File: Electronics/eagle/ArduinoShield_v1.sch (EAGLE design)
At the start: 41 parts, among them IC1 74AC14N, IC3 ACS770LCB-50B

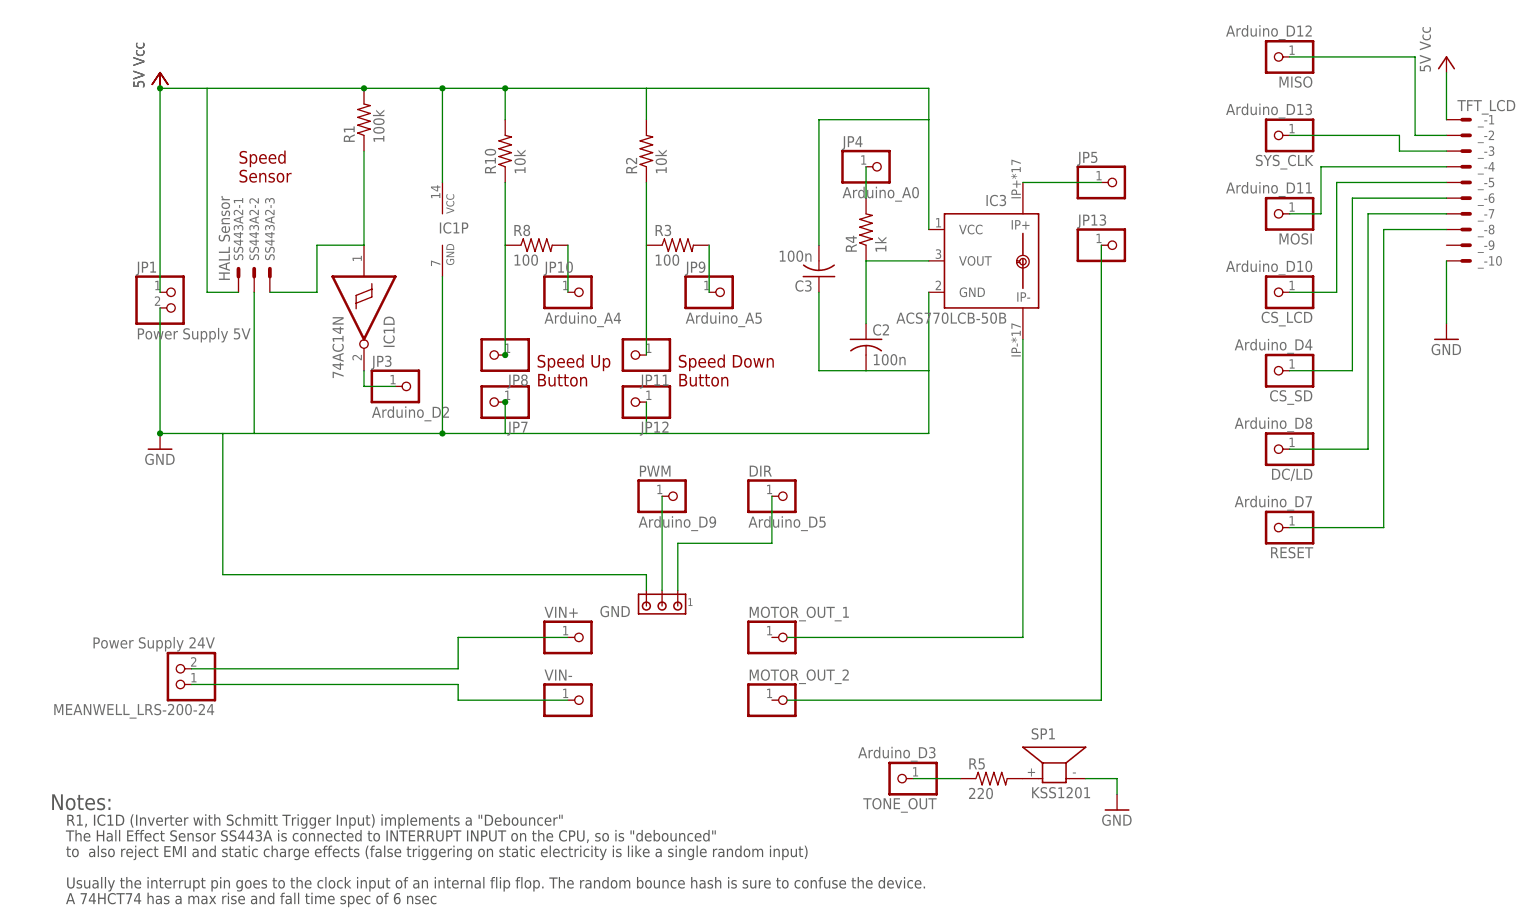
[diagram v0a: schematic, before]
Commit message: Version 0.9
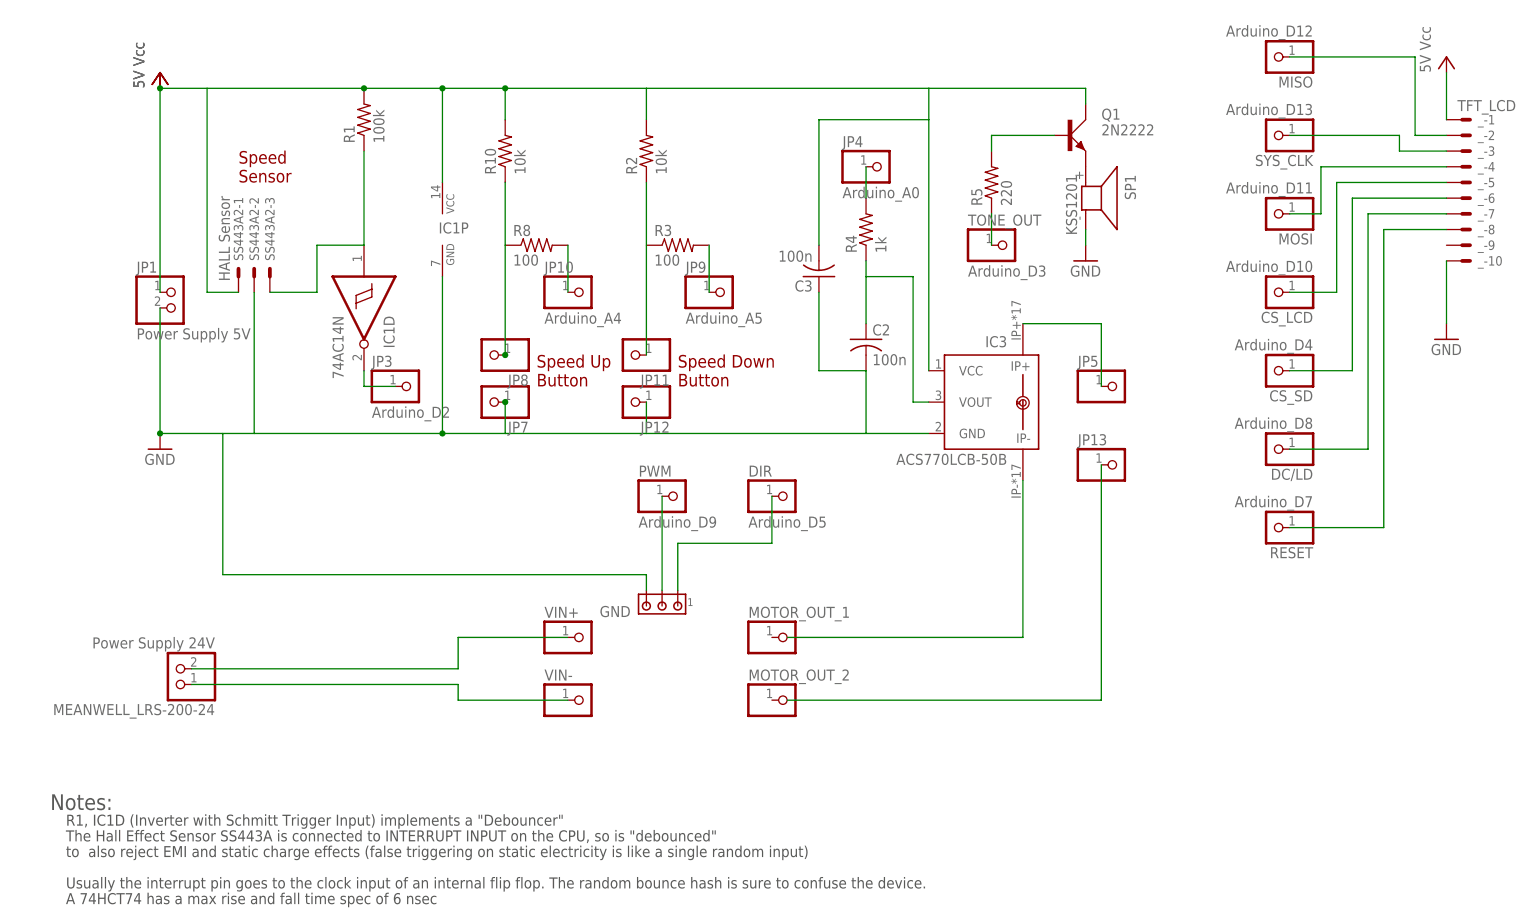
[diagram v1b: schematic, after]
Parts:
- added Q1: 2N2222, transistor-small-signal:2N2222
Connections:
- new net N$23: Q1.B, R5.2
- net N$14: now also Q1.E; no longer R5.2
- net VCC: now also Q1.C
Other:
- moved on the sheet: IC3, JP13, JP5, R5, SP1, TONE_OUT
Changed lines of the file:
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@@
 <part name="RESET" library="pinhead" deviceset="PINHD-1X1" device="" value="Arduino_D7"/>
 <part name="GND3" library="supply1" deviceset="GND" device=""/>
+<part name="Q1" library="transistor-small-signal" deviceset="2N2222" device=""/>
 </parts>
 <sheets>
@@
 <text x="109.22" y="63.5" size="3.81" layer="90">  Motor
 Controller</text>
-<text x="190.5" y="139.7" size="3.81" layer="90" align="center">  Motor
+<text x="190.5" y="106.68" size="3.81" layer="90" align="center">  Motor
 </text>
 </plain>
@@
 <instance part="JP12" gate="G$1" x="114.3" y="111.76" rot="R180"/>
 <instance part="R3" gate="G$1" x="121.92" y="137.16"/>
-<instance part="IC3" gate="G$1" x="172.72" y="134.62" rot="MR0"/>
+<instance part="IC3" gate="G$1" x="172.72" y="111.76" rot="MR0"/>
 <instance part="R4" gate="G$1" x="152.4" y="139.7" rot="R90"/>
 <instance part="JP4" gate="G$1" x="154.94" y="149.86"/>
-<instance part="JP5" gate="G$1" x="193.04" y="147.32"/>
-<instance part="JP13" gate="G$1" x="193.04" y="137.16"/>
+<instance part="JP5" gate="G$1" x="193.04" y="114.3"/>
+<instance part="JP13" gate="G$1" x="193.04" y="101.6"/>
 <instance part="MOTOR_OUT_1" gate="G$1" x="139.7" y="73.66"/>
 <instance part="MOTOR_OUT_2" gate="G$1" x="139.7" y="63.5"/>
@@
 <instance part="PWM" gate="G$1" x="121.92" y="96.52"/>
 <instance part="MEANWELL_LRS-200-24" gate="G$1" x="40.64" y="68.58" rot="R180"/>
-<instance part="SP1" gate="1" x="182.88" y="50.8"/>
+<instance part="SP1" gate="1" x="187.96" y="144.78" rot="R270"/>
 <instance part="P+2" gate="VCC" x="38.1" y="165.1"/>
-<instance part="GND2" gate="1" x="193.04" y="45.72"/>
-<instance part="R5" gate="G$1" x="172.72" y="50.8"/>
-<instance part="TONE_OUT" gate="G$1" x="157.48" y="50.8" rot="R180"/>
+<instance part="GND2" gate="1" x="187.96" y="134.62"/>
+<instance part="R5" gate="G$1" x="172.72" y="147.32" rot="R90"/>
+<instance part="TONE_OUT" gate="G$1" x="175.26" y="137.16"/>
 <instance part="_" gate="-1" x="248.92" y="157.48"/>
 <instance part="_" gate="-2" x="248.92" y="154.94"/>
@@
 <instance part="RESET" gate="G$1" x="218.44" y="91.44" rot="R180"/>
 <instance part="GND3" gate="1" x="246.38" y="121.92"/>
+<instance part="Q1" gate="1" x="185.42" y="154.94"/>
 </instances>
 <busses>
@@
 <wire x1="116.84" y1="157.48" x2="116.84" y2="162.56" width="0.1524" layer="91"/>
 <pinref part="IC3" gate="G$1" pin="VCC"/>
-<wire x1="162.56" y1="139.7" x2="162.56" y2="157.48" width="0.1524" layer="91"/>
+<wire x1="162.56" y1="116.84" x2="162.56" y2="157.48" width="0.1524" layer="91"/>
 <pinref part="C3" gate="G$1" pin="2"/>
 <wire x1="162.56" y1="157.48" x2="162.56" y2="162.56" width="0.1524" layer="91"/>
@@
 <junction x="71.12" y="162.56"/>
 <pinref part="P+2" gate="VCC" pin="VCC"/>
+<wire x1="162.56" y1="162.56" x2="187.96" y2="162.56" width="0.1524" layer="91"/>
+<pinref part="Q1" gate="1" pin="C"/>
+<wire x1="187.96" y1="162.56" x2="187.96" y2="160.02" width="0.1524" layer="91"/>
 </segment>
 <segment>
@@
 <wire x1="83.82" y1="106.68" x2="93.98" y2="106.68" width="0.1524" layer="91"/>
 <wire x1="93.98" y1="106.68" x2="116.84" y2="106.68" width="0.1524" layer="91"/>
-<wire x1="116.84" y1="106.68" x2="162.56" y2="106.68" width="0.1524" layer="91"/>
+<wire x1="116.84" y1="106.68" x2="152.4" y2="106.68" width="0.1524" layer="91"/>
 <pinref part="GND1" gate="1" pin="GND"/>
 <junction x="38.1" y="106.68"/>
 <pinref part="IC1" gate="P" pin="GND"/>
+<wire x1="152.4" y1="106.68" x2="162.56" y2="106.68" width="0.1524" layer="91"/>
 <wire x1="83.82" y1="132.08" x2="83.82" y2="106.68" width="0.1524" layer="91"/>
 <junction x="83.82" y="106.68"/>
@@
 <wire x1="116.84" y1="111.76" x2="116.84" y2="106.68" width="0.1524" layer="91"/>
 <pinref part="IC3" gate="G$1" pin="GND"/>
-<wire x1="162.56" y1="129.54" x2="162.56" y2="116.84" width="0.1524" layer="91"/>
-<pinref part="C2" gate="G$1" pin="2"/>
-<wire x1="162.56" y1="116.84" x2="162.56" y2="106.68" width="0.1524" layer="91"/>
-<wire x1="152.4" y1="116.84" x2="162.56" y2="116.84" width="0.1524" layer="91"/>
-<pinref part="C3" gate="G$1" pin="1"/>
-<wire x1="152.4" y1="116.84" x2="144.78" y2="116.84" width="0.1524" layer="91"/>
-<wire x1="144.78" y1="116.84" x2="144.78" y2="129.54" width="0.1524" layer="91"/>
 <pinref part="GND" gate="G$1" pin="3"/>
 <wire x1="116.84" y1="81.28" x2="116.84" y2="83.82" width="0.1524" layer="91"/>
 <wire x1="116.84" y1="83.82" x2="48.26" y2="83.82" width="0.1524" layer="91"/>
 <wire x1="48.26" y1="83.82" x2="48.26" y2="106.68" width="0.1524" layer="91"/>
+<pinref part="C3" gate="G$1" pin="1"/>
+<pinref part="C2" gate="G$1" pin="2"/>
+<wire x1="152.4" y1="116.84" x2="144.78" y2="116.84" width="0.1524" layer="91"/>
+<wire x1="144.78" y1="116.84" x2="144.78" y2="129.54" width="0.1524" layer="91"/>
+<wire x1="152.4" y1="116.84" x2="152.4" y2="106.68" width="0.1524" layer="91"/>
 </segment>
 <segment>
 <pinref part="SP1" gate="1" pin="2"/>
 <pinref part="GND2" gate="1" pin="GND"/>
-<wire x1="187.96" y1="50.8" x2="193.04" y2="50.8" width="0.1524" layer="91"/>
-<wire x1="193.04" y1="50.8" x2="193.04" y2="48.26" width="0.1524" layer="91"/>
+<wire x1="187.96" y1="139.7" x2="187.96" y2="137.16" width="0.1524" layer="91"/>
 </segment>
 <segment>
@@
 <pinref part="R4" gate="G$1" pin="1"/>
 <pinref part="C2" gate="G$1" pin="1"/>
-<wire x1="152.4" y1="134.62" x2="152.4" y2="124.46" width="0.1524" layer="91"/>
+<wire x1="152.4" y1="134.62" x2="152.4" y2="132.08" width="0.1524" layer="91"/>
+<wire x1="152.4" y1="132.08" x2="152.4" y2="124.46" width="0.1524" layer="91"/>
+<wire x1="152.4" y1="132.08" x2="160.02" y2="132.08" width="0.1524" layer="91"/>
+<wire x1="160.02" y1="132.08" x2="160.02" y2="111.76" width="0.1524" layer="91"/>
 <pinref part="IC3" gate="G$1" pin="VOUT"/>
-<wire x1="162.56" y1="134.62" x2="152.4" y2="134.62" width="0.1524" layer="91"/>
+<wire x1="160.02" y1="111.76" x2="162.56" y2="111.76" width="0.1524" layer="91"/>
 </segment>
 </net>
@@
 <wire x1="139.7" y1="73.66" x2="177.8" y2="73.66" width="0.1524" layer="91"/>
 <pinref part="IC3" gate="G$1" pin="IP-"/>
-<wire x1="177.8" y1="73.66" x2="177.8" y2="121.92" width="0.1524" layer="91"/>
+<wire x1="177.8" y1="73.66" x2="177.8" y2="99.06" width="0.1524" layer="91"/>
 </segment>
 </net>
@@
 <pinref part="JP13" gate="G$1" pin="1"/>
 <wire x1="139.7" y1="63.5" x2="190.5" y2="63.5" width="0.1524" layer="91"/>
-<wire x1="190.5" y1="63.5" x2="190.5" y2="137.16" width="0.1524" layer="91"/>
-</segment>
-</net>
-<net name="N$4" class="0">
-<segment>
-<pinref part="IC3" gate="G$1" pin="IP+"/>
-<pinref part="JP5" gate="G$1" pin="1"/>
-<wire x1="177.8" y1="147.32" x2="190.5" y2="147.32" width="0.1524" layer="91"/>
-</segment>
-</net>
-<net name="N$14" class="0">
-<segment>
-<pinref part="SP1" gate="1" pin="1"/>
-<pinref part="R5" gate="G$1" pin="2"/>
+<wire x1="190.5" y1="63.5" x2="190.5" y2="101.6" width="0.1524" layer="91"/>
 </segment>
 </net>
@@
 <pinref part="TONE_OUT" gate="G$1" pin="1"/>
 <pinref part="R5" gate="G$1" pin="1"/>
-<wire x1="160.02" y1="50.8" x2="167.64" y2="50.8" width="0.1524" layer="91"/>
+<wire x1="172.72" y1="137.16" x2="172.72" y2="142.24" width="0.1524" layer="91"/>
 </segment>
 </net>
@@
 </segment>
 </net>
+<net name="N$4" class="0">
+<segment>
+<pinref part="JP5" gate="G$1" pin="1"/>
+<wire x1="190.5" y1="114.3" x2="190.5" y2="124.46" width="0.1524" layer="91"/>
+<pinref part="IC3" gate="G$1" pin="IP+"/>
+<wire x1="190.5" y1="124.46" x2="177.8" y2="124.46" width="0.1524" layer="91"/>
+</segment>
+</net>
+<net name="N$14" class="0">
+<segment>
+<pinref part="SP1" gate="1" pin="1"/>
+<pinref part="Q1" gate="1" pin="E"/>
+</segment>
+</net>
+<net name="N$23" class="0">
+<segment>
+<pinref part="R5" gate="G$1" pin="2"/>
+<wire x1="172.72" y1="152.4" x2="172.72" y2="154.94" width="0.1524" layer="91"/>
+<pinref part="Q1" gate="1" pin="B"/>
+<wire x1="172.72" y1="154.94" x2="182.88" y2="154.94" width="0.1524" layer="91"/>
+</segment>
+</net>
